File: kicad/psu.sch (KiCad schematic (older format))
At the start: 14 parts

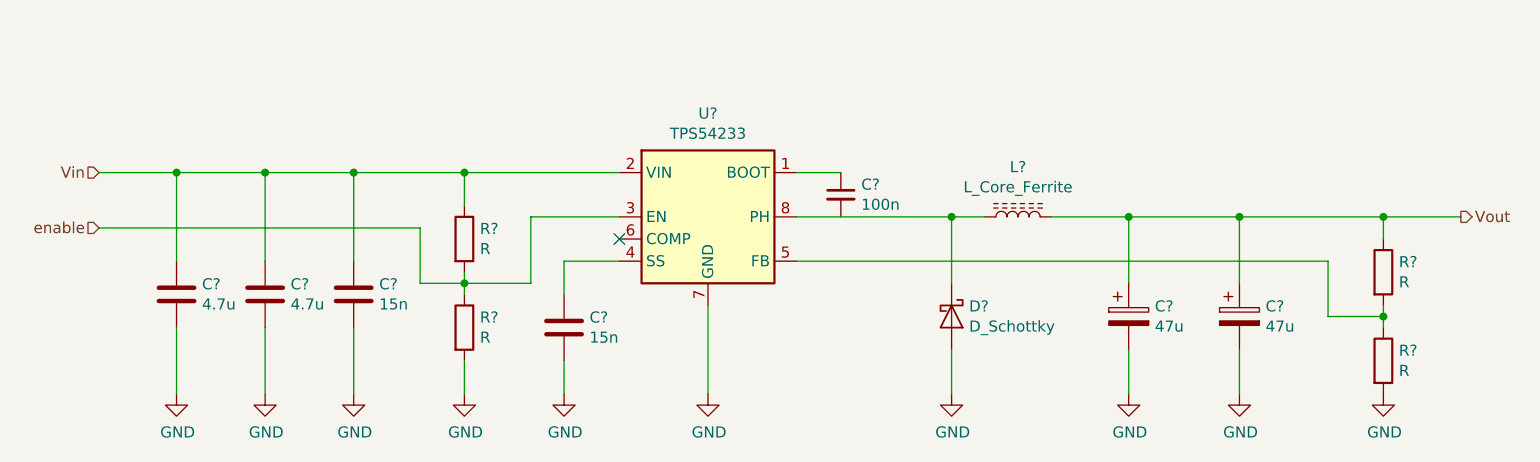
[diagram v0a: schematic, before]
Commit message: z
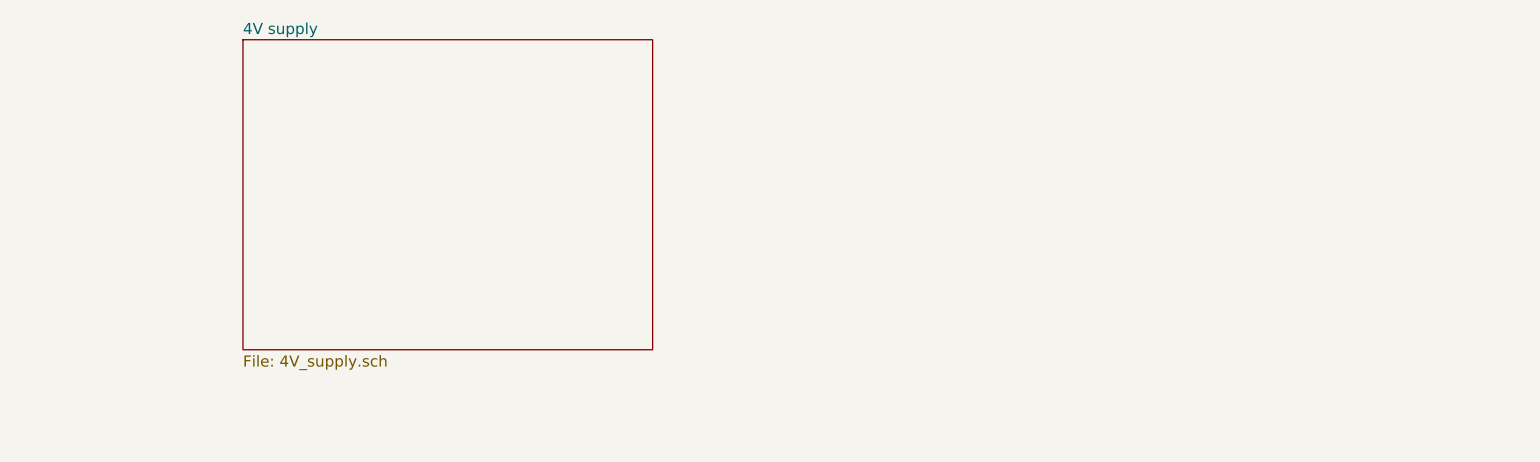
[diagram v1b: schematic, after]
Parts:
- removed C? (x2): 15n, symbol Device:C
- removed C? (x2): 4.7u, symbol Device:C
- removed C?: 100n, symbol Device:C_Small
- removed C? (x2): 47u, symbol Device:CP
- removed D?: D_Schottky, symbol Device:D_Schottky
- removed L?: L_Core_Ferrite, symbol Device:L_Core_Ferrite
- removed R? (x4): R, symbol Device:R
- removed U?: TPS54233, Package_SO:SOIC-8_3.9x4.9mm_P1.27mm, symbol Regulator_Switching:TPS54233
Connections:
- no-connect marks 1 -> 0
